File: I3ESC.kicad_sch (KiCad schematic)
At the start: 56 parts, among them J10 VIN_BARREL, J5 Encoder1, J7 VIN_TERMINAL, J8 Encoder2, SW1 reset, SW2 boot-red, SW3 user1-white, U1 SY8113BADC, U11 Qwiic2, U3 SPX3819M5-L-3-3, U4 STM32G474RETx, U5 Qwiic1, U7 Prog, U8 ABM3B-8.000MHZ

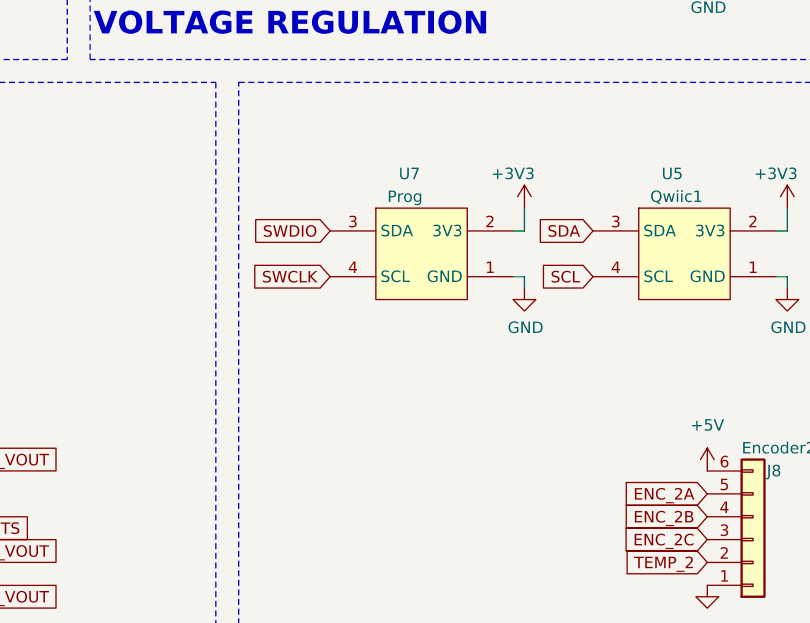
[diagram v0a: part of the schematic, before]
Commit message: updates for production run 2
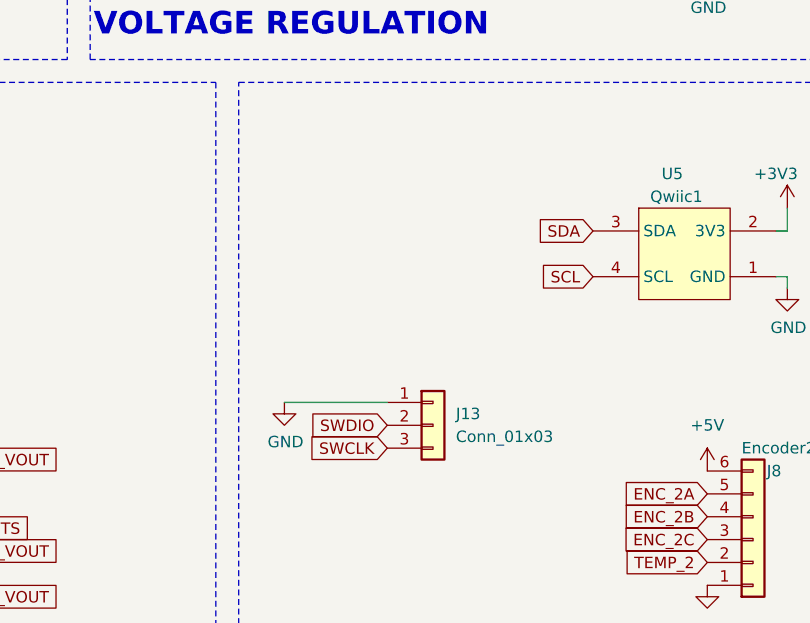
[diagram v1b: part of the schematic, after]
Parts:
- removed U7: Prog, Connector_JST:JST_SH_BM04B-SRSS-TB_1x04-1MP_P1.00mm_Vertical, symbol AlfredoSymbols:QwiicConnector
- added J13: Conn_01x03, AlfredoFootprints:PinHeader_1x03_P2.54mm_Vertical, symbol Connector_Generic:Conn_01x03
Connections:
- net GND: now also J13.1 (Pin_1)
- net SWCLK: now also J13.3 (Pin_3)
- net SWDIO: now also J13.2 (Pin_2)
